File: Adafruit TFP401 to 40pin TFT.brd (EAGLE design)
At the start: 66 x 50.8 mm, 92 parts, among them IC1 AR1100_SSOP, Q1 BSS138, U1 TFP401, U2 24LC02BT-I/OT, U3 LT1117(3V3), U4 FAN5333BSX, X1 47151-0001, X2 microUSB, X3 XF2-40-RARBT, Y1 12MHz

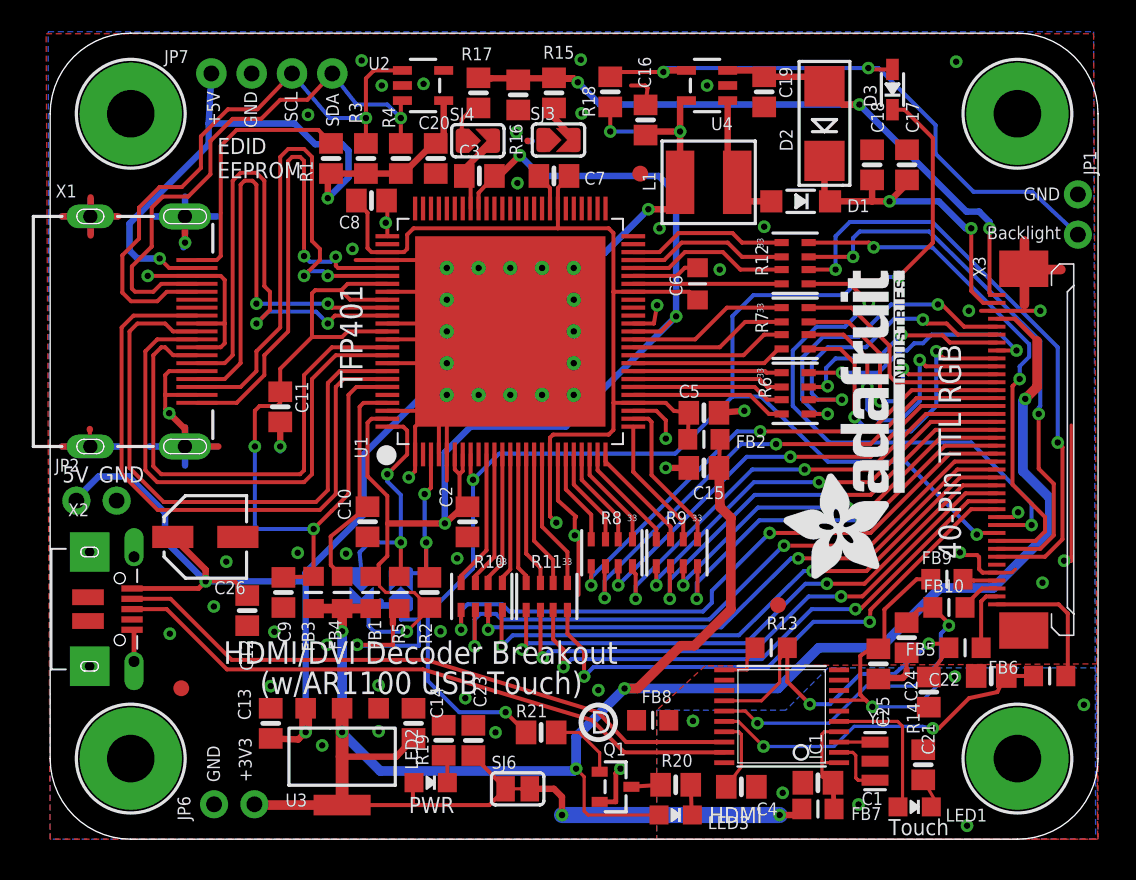
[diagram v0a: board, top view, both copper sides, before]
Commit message: Модификация платы
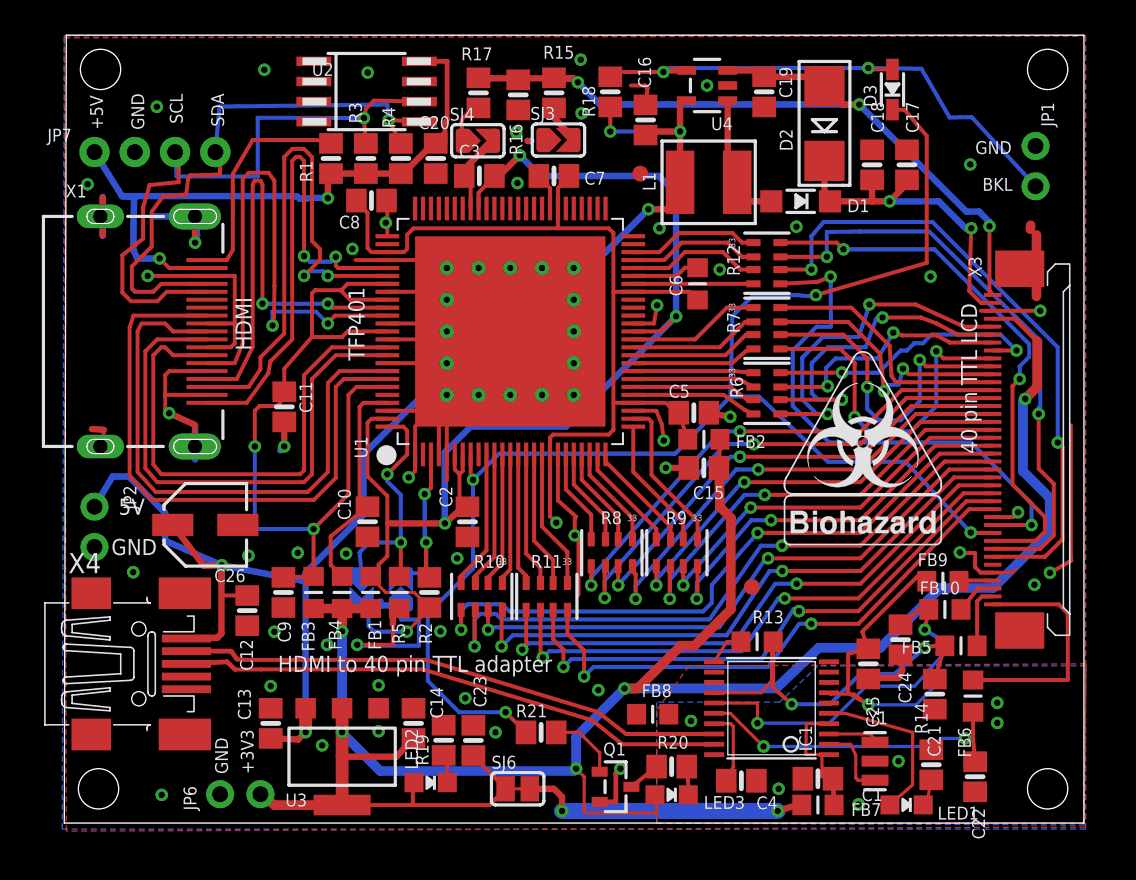
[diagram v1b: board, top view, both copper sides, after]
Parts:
- removed FID2: FIDUCIAL"", microbuilder:FIDUCIAL_1MM
- removed U$80: (no value), microbuilder:PCBFEAT-REV-056
- removed U$81: (no value), microbuilder:ADAFRUIT_TEXT_20MM
- removed X2: microUSB, microbuilder:4UCONN_20329
- added U$35: (no value), logo:BIOHAZARD_10.00
- added X4: MINI-USB-32005-201, con-cypressindustries:32005-201
- U$31, U$32, U$33, U$34: value MOUNTINGHOLE3.0 -> (none); device microbuilder:MOUNTINGHOLE_3.0_PLATED -> special-drill:DRILL_0.1000
- U2: device microbuilder:SOT23-5 -> microchip:SO-08M
- moved U$31 71.8 mm to (62.9, 3.17)
- moved U$33 57.9 mm to (3.05, 3.17)
- moved U$34 43.5 mm to (3.17, 48.5)
- moved JP7 8.88 mm to (6.60, 43.3)
- moved C22 6.43 mm to (58.3, 3.94), turned to 270 degrees
- moved FB6 4.99 mm to (58.2, 9.02), turned to 90 degrees
- moved JP1 4.05 mm to (62.1, 42.4)
- moved U2 3.58 mm to (19.9, 47.1)
- moved U$32 3.38 mm to (62.9, 48.5)
- moved FID3 2.01 mm to (44.2, 15.9)
- moved R12 1.78 mm to (45.2, 36.3)
- moved R6 1.78 mm to (45.2, 28.1)
- moved R7 1.78 mm to (45.2, 32.2)
- moved JP2 1.66 mm to (2.79, 19.7), turned to 270 degrees
- moved LED3 1.30 mm to (39.2, 2.80)
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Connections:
- net 5.0V: now also U2.8; no longer U2.4
- net D+: now also X4.3; no longer X2.D+
- net D-: now also X4.2; no longer X2.D-
- net GND: now also U2.4, U2.7, X4.5; no longer U2.2, U2.5, X2.BASE@1, X2.BASE@2, X2.GND, X2.SPRT@1, X2.SPRT@2, X2.SPRT@3, X2.SPRT@4
- net SCL: now also U2.6; no longer U2.1
- net SDA: now also U2.5; no longer U2.3
- net VIN: now also X4.1; no longer X2.VBUS
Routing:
- net N$54: track 8.70 -> 15.1 mm
- net D-: track 40.2 -> 34.5 mm
- net D+: track 40.2 -> 34.5 mm
- net GND: track 182.4 -> 177.3 mm
- net N$52: track 38.1 -> 33.8 mm
- net VIN: track 96.4 -> 100.0 mm
- net SCL: track 37.9 -> 40.2 mm
- net VSYNC: track 35.4 -> 37.7 mm
- net Y+: track 21.6 -> 23.8 mm
- net X+: track 18.0 -> 20.2 mm
- net DISPEN: track 38.3 -> 40.3 mm
- net N$9: track 16.3 -> 14.3 mm
- net N$17: track 15.7 -> 17.8 mm
- net HSYNC: track 32.9 -> 35.0 mm
- net N$15: track 19.3 -> 21.2 mm
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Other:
- board size 66 x 50.8 mm -> 64.3 x 49.7 mm
- board text added: "40 pin TTL LCD"
- board text added: "BKL"
- board text added: "HDMI to 40 pin TTL adapter"
- board text removed: "(w/AR1100 USB Touch)"
- board text removed: "40-Pin TTL RGB"
- board text removed: "Backlight"
- board text removed: "EDID EEPROM"
- board text removed: "HDMI/DVI Decoder Breakout"
- board text removed: "PWR"
- board text removed: "Touch"
